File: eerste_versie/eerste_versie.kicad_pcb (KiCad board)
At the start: 2 copper layers, 16 parts, among them U1 ESP32-WROOM-32U, U2 AMS1117-3.3, X1 DG3XX-02-5.0

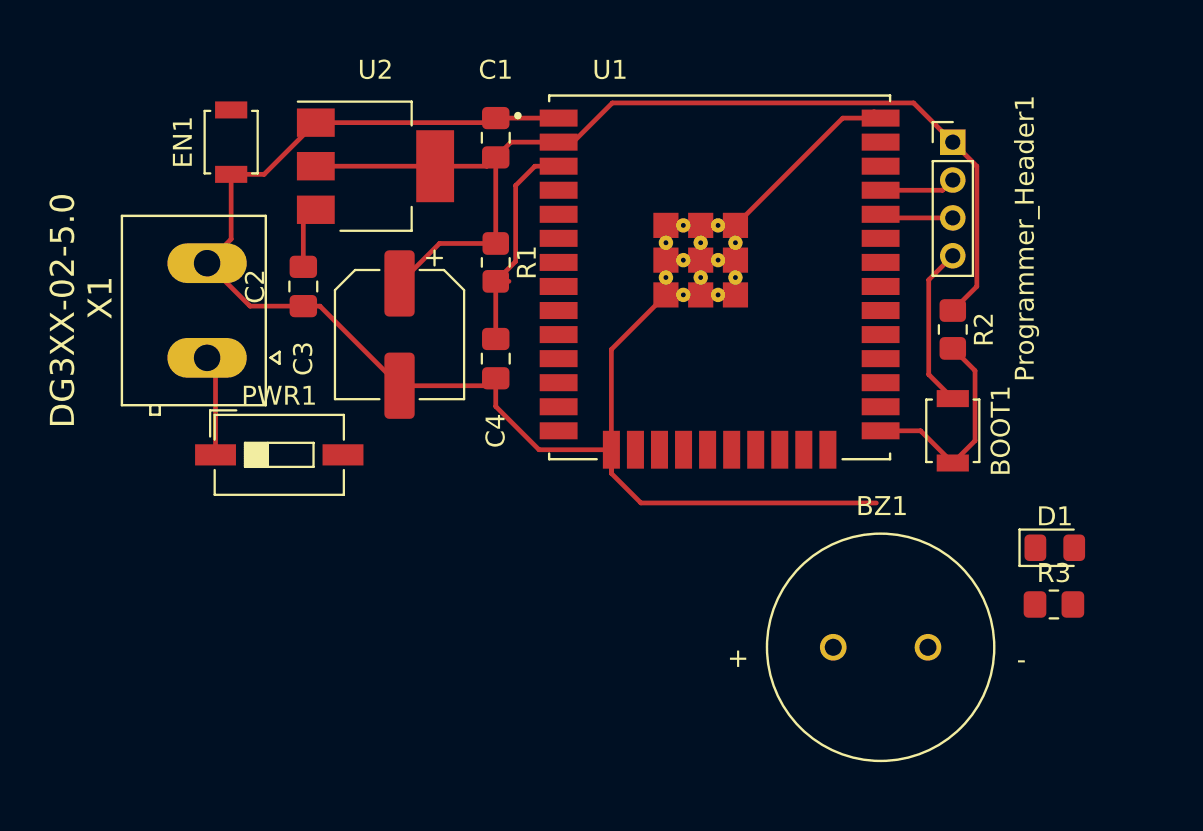
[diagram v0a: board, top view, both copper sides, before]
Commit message: derde_versie
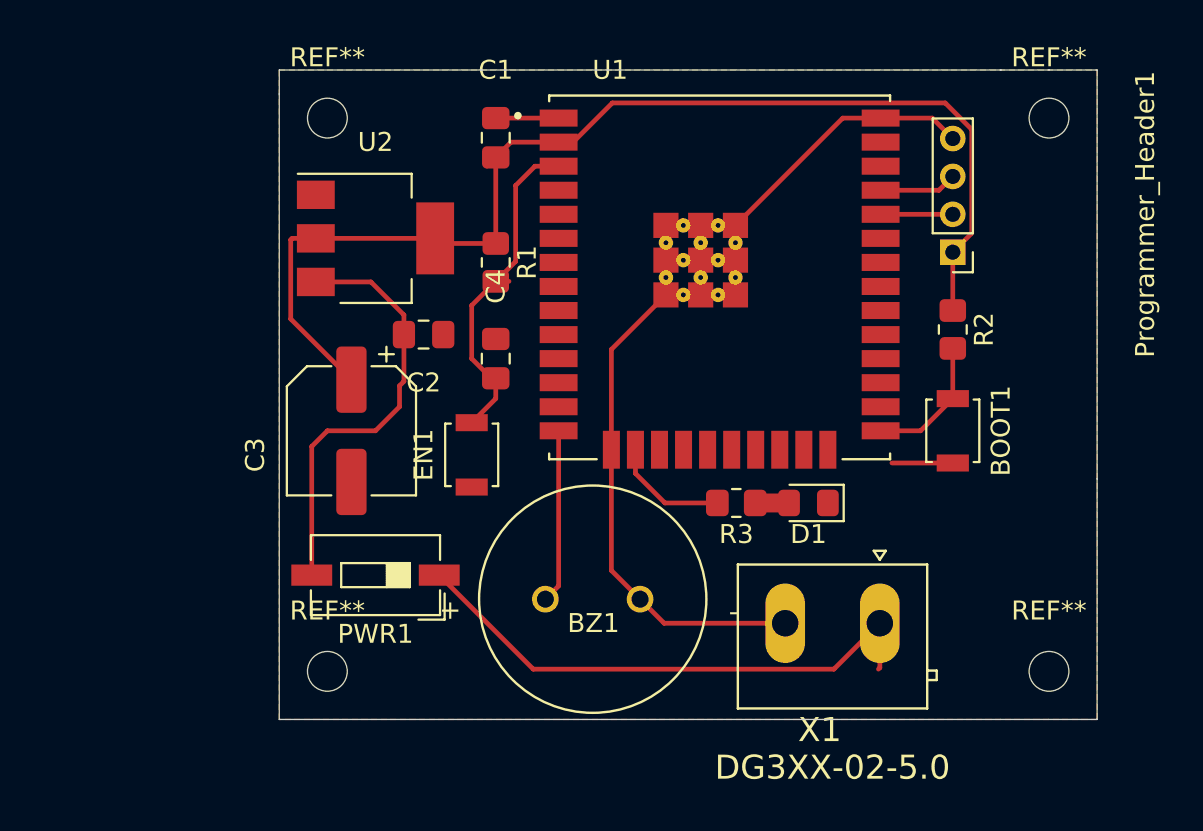
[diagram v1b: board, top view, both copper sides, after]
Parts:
- added REF**: MountingHole_2.1mm, MountingHole:MountingHole_2.1mm, F.Cu at (157.5, 135.9)
- added REF**: MountingHole_2.1mm, MountingHole:MountingHole_2.1mm, F.Cu at (119.4, 106.7)
- added REF**: MountingHole_2.1mm, MountingHole:MountingHole_2.1mm, F.Cu at (157.5, 106.7)
- added REF**: MountingHole_2.1mm, MountingHole:MountingHole_2.1mm, F.Cu at (119.4, 135.9)
- moved X1 36.9 mm to (146.1, 133.3), turned to 180 degrees
- moved EN1 20.8 mm to (127.0, 124.5)
- moved R3 17.6 mm to (141.0, 127.0), turned to 180 degrees
- moved BZ1 15.4 mm to (133.4, 132.1)
- moved D1 13.2 mm to (144.8, 127.0), turned to 180 degrees
- moved PWR1 8.13 mm to (121.9, 130.8), turned to 180 degrees
- moved C2 6.84 mm to (124.5, 118.1), turned to 0 degrees
- moved Programmer_Header1 5.81 mm to (152.4, 113.8), turned to 180 degrees
- moved C3 5.68 mm to (120.7, 123.2)
- moved U2 3.81 mm to (121.9, 113.0)
- turned BOOT1 to 270 degrees
- turned C4 to 90 degrees
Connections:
- U1 pad 34: Net-(Programmer_Header1-Pad3) -> Net-(Programmer_Header1-Pad2)
- U1 pad 35: Net-(Programmer_Header1-Pad2) -> Net-(Programmer_Header1-Pad3)
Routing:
- net GND: track 118.2 -> 69.6 mm
- net Net-(PWR1-Pad1): track 5.30 -> 29.4 mm
- net Net-(C2-Pad1): track 3.89 -> 23.2 mm
- net Net-(BZ1-Pad1): track 0.00 -> 9.18 mm
- net Net-(R3-Pad2): track 0.00 -> 6.22 mm
- net Net-(C4-Pad1): track 12.7 -> 18.9 mm
- net Net-(BOOT1-Pad1): track 12.3 -> 7.93 mm
- net VDD33: track 57.6 -> 62.0 mm
- net Net-(D1-Pad2): track 0.00 -> 1.78 mm
- added copper zone on F.Cu, net GND
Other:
- board outline added: 43.2 x 34.3 mm

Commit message: volledige versie
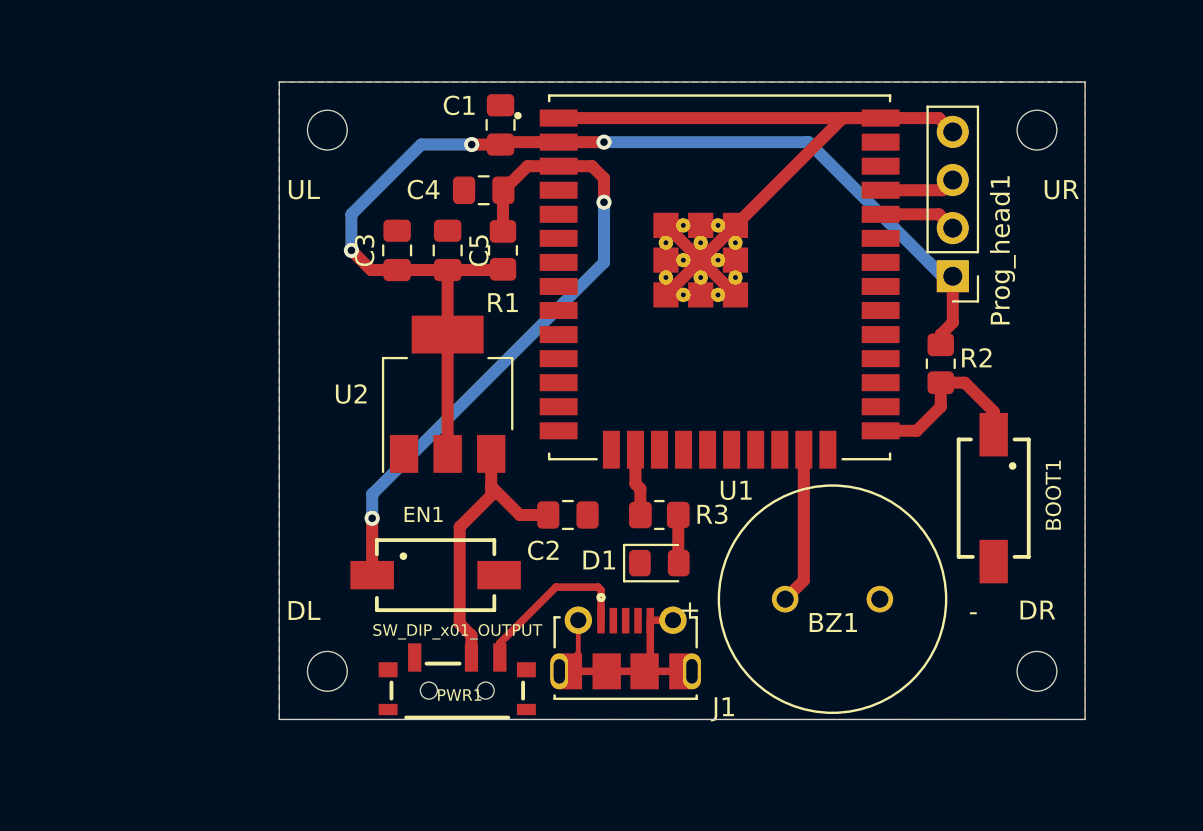
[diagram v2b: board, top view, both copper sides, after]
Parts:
- removed X1: DG3XX-02-5.0, degson:degson-DG306-5.0-02P
- added C5: 100n, Capacitor_SMD:C_0805_2012Metric_Pad1.18x1.45mm_HandSolder, F.Cu at (125.7, 113.7)
- added J1: 105017-1001, 105017-1001:MOLEX_105017-1001, F.Cu at (135.1, 135.9)
- BOOT1, EN1: footprint Button_Switch_SMD:SW_SPST_B3U-1000P -> 434111043826:434111043826
- C2: value 100n -> 10uF
- C3: value 47u -> 10uF; footprint Capacitor_SMD:CP_Elec_6.3x3 -> Capacitor_SMD:C_0805_2012Metric_Pad1.18x1.45mm_HandSolder
- PWR1: footprint Button_Switch_SMD:SW_DIP_SPSTx01_Slide_6.7x4.1mm_W6.73mm_P2.54mm_LowProfile_JPin -> sparkfun:SWITCH_SPST_SMD_A
- Prog_head1: renamed from Programmer_Header1; footprint Connector_PinHeader_2.00mm:PinHeader_1x04_P2.00mm_Vertical -> Connector_PinHeader_2.54mm:PinHeader_1x04_P2.54mm_Vertical
- moved BZ1 12.7 mm to (146.1, 132.1)
- moved C2 12.2 mm to (132.1, 127.6)
- moved C3 9.83 mm to (123.1, 113.7), turned to 90 degrees
- moved U2 9.07 mm to (125.7, 121.3), turned to 90 degrees
- moved C4 8.91 mm to (127.6, 110.5), turned to 180 degrees
- moved D1 8.49 mm to (136.9, 130.2), turned to 0 degrees
- moved PWR1 7.47 mm to (126.2, 136.9)
- moved EN1 6.63 mm to (125.1, 130.8), turned to 0 degrees
- moved BOOT1 4.16 mm to (154.6, 126.7)
- moved R3 4.11 mm to (136.9, 127.6)
- moved R2 1.92 mm to (151.8, 119.7)
- moved Prog_head1 1.27 mm to (152.4, 115.0)
- moved UR 0.90 mm to (156.8, 107.3)
- moved R1 0.74 mm to (128.7, 113.7), turned to 90 degrees
- moved C1 0.72 mm to (128.5, 107.0)
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- renumbered REF** to DL, REF** to DR, REF** to UL, REF** to UR
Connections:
- U1 pad 14: Net-(BZ1-Pad1) -> Net-(U1-Pad14)
- U1 pad 23: Net-(U1-Pad23) -> Net-(BZ1-Pad1)
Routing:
- net Net-(J1-Pad1): track 29.4 -> 9.00 mm
- net Net-(C4-Pad1): track 18.9 -> 34.3 mm, vias 0 -> 2
- net GND: track 69.6 -> 77.6 mm
- net Net-(C2-Pad1): track 23.2 -> 16.0 mm
- net Net-(R3-Pad2): track 6.22 -> 3.55 mm
- net Net-(BOOT1-Pad1): track 7.93 -> 9.62 mm
- net VDD33: track 62.0 -> 60.8 mm, vias 0 -> 3
- net Net-(BZ1-Pad1): track 9.18 -> 8.30 mm
- net Net-(D1-Pad2): track 1.78 -> 2.55 mm
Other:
- board size 43.2 x 34.3 mm -> 42.5 x 33.7 mm
- net class Default: trace_width 0.25 -> 0.254
- rule trace_min: 0.2 -> 0.1524
